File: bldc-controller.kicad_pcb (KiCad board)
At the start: 2 copper layers, 47 x 39 mm, 98 parts, among them IC1 L6205PD, P1 CON_LED, P10 MOUNTING, P11 CONN_01X03, P12 CONN_01X03, P2 MOUNTING, P3 CON_MOTOR, P4 USB_OTG, P5 CON_SWD, P6 CON_HALL, P7 CON_PWR_BRD, P8 MOUNTING, P9 MOUNTING, U1 STM32F405R, U5 MPU6000, U7 LD1117S33TR, Y1 Crystal

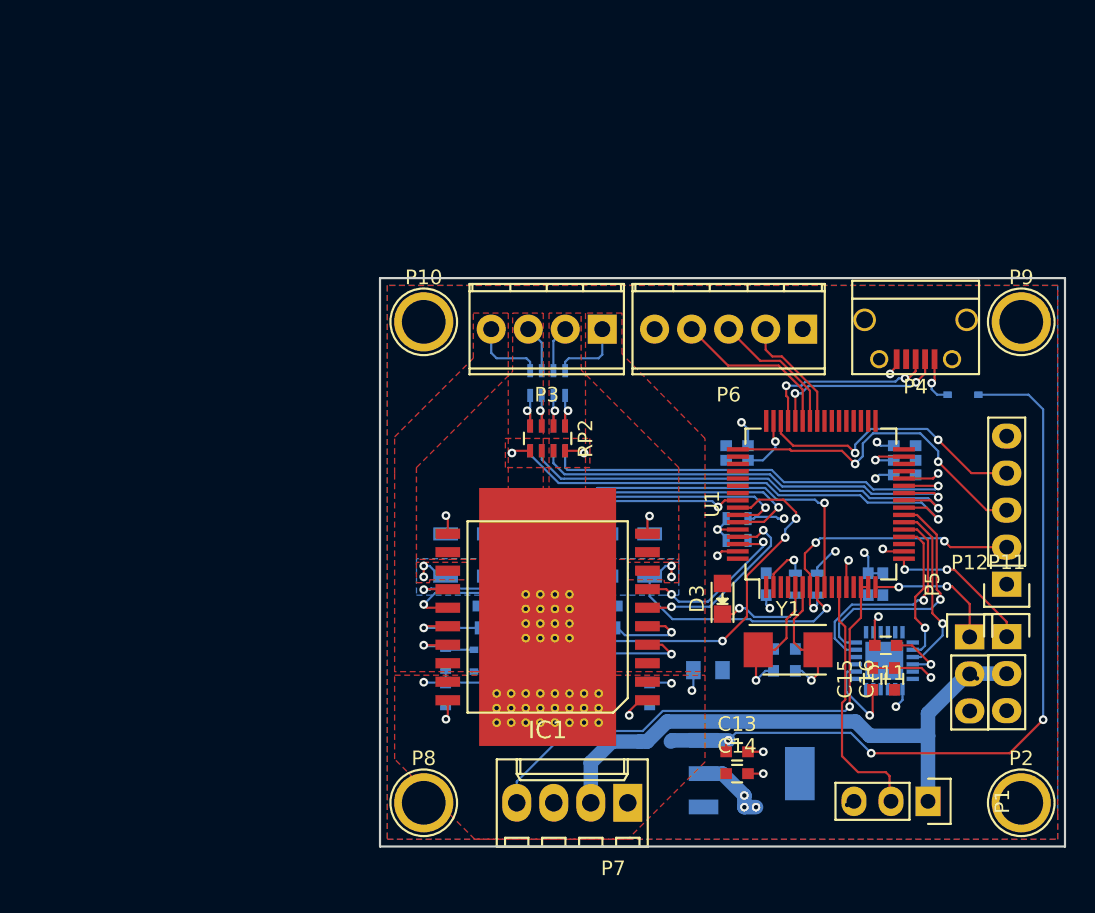
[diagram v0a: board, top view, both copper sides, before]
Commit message: routed... at least for now
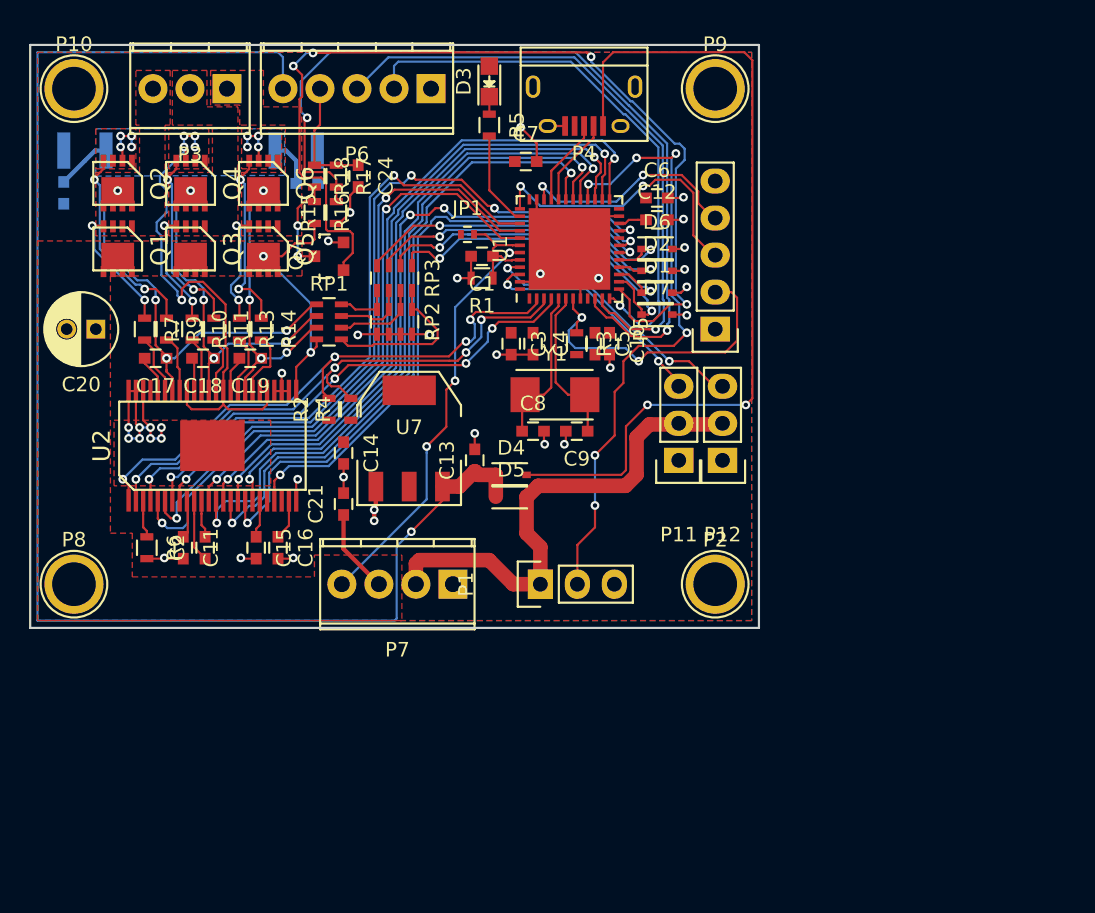
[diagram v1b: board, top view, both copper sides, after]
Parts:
- removed D8: D, Diodes_SMD:SOD-323
- removed IC1: L6205PD, BLDC:SOIC-20
- removed REF**1111111, REF**11111111111, REF**11111111112, REF**11111111113, REF**11111111114, REF**11111111121, REF**11111111122, REF**11111111123, REF**11111111124, REF**11111111131, REF**11111111132, REF**11111111133, REF**11111111134, REF**11111111141, REF**11111111142, REF**11111111143, REF**11111111144, REF**1111112, REF**1111113, REF**1111121, REF**1111122, REF**1111123, REF**1111131, REF**1111132, REF**1111133, REF**1111141, REF**1111142, REF**1111143, REF**1111151, REF**1111152, REF**1111153, REF**1111161, REF**1111162, REF**1111163, REF**1111171, REF**1111172, REF**1111173, REF**1111181, REF**1111182, REF**1111183: VIA-0.6, BLDC:VIA-0.6
- removed U5: MPU6000, Housings_DFN_QFN:QFN-24-1EP_4x4mm_Pitch0.5mm
- added C23: 1nF, Capacitors_SMD:C_0603, B.Cu at (119.0, 59.5)
- added C24: NA/100nF, Capacitors_SMD:C_0603, F.Cu at (122.5, 59.0)
- added D5: D_Small, Diodes_SMD:SOD-323, F.Cu at (133.0, 81.0)
- added D6: 3.3V, Diodes_SMD:SOD-323, F.Cu at (143.0, 64.0)
- added D7: 3.3V, Diodes_SMD:SOD-323, F.Cu at (143.0, 68.5)
- added JP1: OPEN, Resistors_SMD:R_0402, F.Cu at (130.0, 63.0)
- added Q1: Q_NMOS_DGS, BLDC:SOT1210, F.Cu at (106.0, 64.0)
- added Q2: Q_NMOS_DGS, BLDC:SOT1210, F.Cu at (106.0, 59.5)
- added Q3: Q_NMOS_DGS, BLDC:SOT1210, F.Cu at (111.0, 64.0)
- added Q4: Q_NMOS_DGS, BLDC:SOT1210, F.Cu at (111.0, 59.5)
- added Q5: Q_NMOS_DGS, BLDC:SOT1210, F.Cu at (116.0, 64.0)
- added Q6: Q_NMOS_DGS, BLDC:SOT1210, F.Cu at (116.0, 59.5)
- added Q7: 2N7002, TO_SOT_Packages_SMD:SOT-23, F.Cu at (120.5, 64.5)
- added R12: .01, Resistors_SMD:R_1210, B.Cu at (103.8, 57.2)
- added R13: 10R, Resistors_SMD:R_0603, F.Cu at (114.3, 69.5)
- added R14: 10R, Resistors_SMD:R_0603, F.Cu at (115.8, 69.5)
- added R15: NA/10kR, Resistors_SMD:R_0603, F.Cu at (121.0, 61.5)
- added R16: NA/10kR, Resistors_SMD:R_0603, F.Cu at (119.5, 61.5)
- added R17: 0R/50kR, Resistors_SMD:R_0603, F.Cu at (121.0, 59.0)
- added R18: NA/50kR, Resistors_SMD:R_0603, F.Cu at (119.5, 59.0)
- added U2: DRV8313, BLDC:SOIC-48, F.Cu at (112.5, 77.5)
- C1: value 220nF -> 100nF; moved to F.Cu
- C10, C12, C21, C3, C4, C5, C6, C7, C8, C9, D4, R5, U7: moved to F.Cu
- C11: value 100nF -> 2.2uF
- C17: value 2.2uF -> 100nF; moved to F.Cu
- C18, C19: value 2nF -> 100nF; moved to F.Cu
- C2: value 10nF -> 22nF; moved to F.Cu
- C20: value 100nF -> 10uF; footprint Capacitors_SMD:C_0603 -> Capacitors_ThroughHole:C_Radial_D5_L11_P2; moved to F.Cu
- C22: value 4.7uF -> 1nF; footprint Capacitors_SMD:C_0805 -> Capacitors_SMD:C_0603
- D1, D2: value D_Small -> 3.3V; moved to F.Cu
- P3: value CON_MOTOR -> CONN_01X03; footprint Terminal_Blocks:TerminalBlock_Pheonix_MPT-2.54mm_4pol -> Terminal_Blocks:TerminalBlock_Pheonix_MPT-2.54mm_3pol
- P7: footprint Connectors_Molex:Molex_KK-6410-04_04x2.54mm_Straight -> Terminal_Blocks:TerminalBlock_Pheonix_MPT-2.54mm_4pol
- R1: value 100 -> 10kR; moved to F.Cu
- R10, R11, R9: value .1 -> 10R; footprint Resistors_SMD:R_1206 -> Resistors_SMD:R_0603; moved to F.Cu
- R2: value NA -> 10kR; moved to F.Cu
- R3: value 0 -> 10kR; moved to F.Cu
- R4: value 10k -> 10kR; moved to F.Cu
- R6: value 10k -> 1R; moved to F.Cu
- R7: value 10k -> 10R; moved to F.Cu
- R8: value .1 -> .01; footprint Resistors_SMD:R_1206 -> Resistors_SMD:R_1210
- RP1: value 10k -> 20k; moved to F.Cu
- RP3: value 1k -> 10k; moved to F.Cu
- U1: value STM32F405R -> STM32F401CBUx; footprint Housings_QFP:TQFP-64_10x10mm_Pitch0.5mm -> Housings_DFN_QFN:QFN-48-1EP_7x7mm_Pitch0.5mm
- moved C22 55.0 mm to (102.3, 60.1), turned to 90 degrees
- moved C11 48.7 mm to (110.5, 84.5), turned to 270 degrees
- moved C20 45.5 mm to (104.5, 69.5), turned to 180 degrees
- moved C15 43.2 mm to (115.5, 84.5), turned to 270 degrees
- moved C16 43.2 mm to (117.0, 84.5), turned to 270 degrees
- moved C17 40.5 mm to (108.6, 71.5)
- moved D3 38.9 mm to (131.5, 52.5)
- moved R5 37.9 mm to (131.5, 55.5), turned to 270 degrees
- moved C7 37.3 mm to (134.0, 58.0), turned to 0 degrees
- moved R10 35.0 mm to (111.1, 69.5), turned to 270 degrees
- moved C14 34.8 mm to (121.5, 78.0), turned to 270 degrees
- moved R4 34.2 mm to (122.0, 75.0), turned to 90 degrees
- moved U7 32.9 mm to (126.0, 77.0), turned to 0 degrees
- moved R6 32.0 mm to (108.0, 84.5), turned to 270 degrees
- moved D4 31.5 mm to (133.0, 79.5), turned to 0 degrees
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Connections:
- net /OSC/OSC_IN renamed /OSC_IN
- net /OSC/OSC_OUT renamed /OSC_OUT
- C1 pad 1: Net-(C1-Pad1) -> /BOOT
- C1 pad 2: VPP -> GND
- C16 pad 1: VCC -> Net-(C16-Pad1)
- C17 pad 1: Net-(C17-Pad1) -> /DRV_OUT_1
- C17 pad 2: GND -> Net-(C17-Pad2)
- C18 pad 1: Net-(C18-Pad1) -> /DRV_OUT_2
- C18 pad 2: GND -> Net-(C18-Pad2)
- C19 pad 1: Net-(C19-Pad1) -> /DRV_OUT_3
- C19 pad 2: GND -> Net-(C19-Pad2)
- C22 pad 1: VPP -> GND
- C22 pad 2: GND -> Net-(C22-Pad2)
- D1 pad 1: Net-(D1-Pad1) -> /SENSE_V_3
- D1 pad 2: VPP -> GND
- D2 pad 1: Net-(C1-Pad1) -> /SENSE_V_2
- D2 pad 2: Net-(D1-Pad1) -> GND
- P1 pad 2: /CON_LED/LED_DATA -> /LED_MOSI
- P11 pad 1: /2CON/SIG_1 -> GND
- P11 pad 3: GND -> /PWM_2
- P12 pad 1: /2CON/SIG_2 -> GND
- P12 pad 3: GND -> /PWM_1
- P3 pad 1: /CON_MOTOR/C -> /DRV_OUT_3
- P3 pad 2: /CON_MOTOR/A -> /DRV_OUT_2
- P3 pad 3: /CON_MOTOR/B -> /DRV_OUT_1
- P4 pad 2: /USB/USB_DM -> /USB_D-
- P4 pad 3: /USB/USB_DP -> /USB_D+
- P5 pad 2: /SWDIO/NRST -> /NRST
- P5 pad 3: /SWDIO/SWDCLK -> /SWDCLK
- P5 pad 4: /SWDIO/SWDIO -> /SWDIO
- P6 pad 2: /HALL/HALL_W -> /HALL_W
- P6 pad 3: /HALL/HALL_V -> /HALL_V
- P6 pad 4: /HALL/HALL_U -> Net-(C24-Pad1)
- P6 pad 5: VCC -> +5V
- P7 pad 4: /Power/RX_TX_PWR_BOARD -> /COM_RX_TX_1
- R1 pad 1: Net-(C2-Pad2) -> /BOOT
- R1 pad 2: Net-(D1-Pad1) -> GND
- R10 pad 1: /driver/SENSE_A -> Net-(Q3-Pad2)
- R10 pad 2: GND -> Net-(R10-Pad2)
- R11 pad 1: /driver/SENSE_A -> Net-(Q4-Pad2)
- R11 pad 2: GND -> Net-(R11-Pad2)
- R2 pad 2: Net-(R2-Pad2) -> /DRV_NOCTW
- R3 pad 1: Net-(R2-Pad2) -> /NRST
- R3 pad 2: GND -> VCC
- R4 pad 2: /SWDIO/NRST -> /DRV_NFAULT
- R6 pad 1: Net-(C19-Pad1) -> Net-(R6-Pad1)
- R6 pad 2: /driver/EN_A -> GND
- R7 pad 1: Net-(C18-Pad1) -> Net-(Q1-Pad2)
- R7 pad 2: /driver/EN_B -> Net-(R7-Pad2)
- R8 pad 1: /driver/SENSE_B -> Net-(C22-Pad2)
- R9 pad 1: /driver/SENSE_B -> Net-(Q2-Pad2)
- R9 pad 2: GND -> Net-(R9-Pad2)
- RP1 pad 1: /CON_MOTOR/D -> /DRV_OUT_1
- RP1 pad 2: /CON_MOTOR/B -> /DRV_OUT_2
- RP1 pad 3: /CON_MOTOR/A -> /DRV_OUT_3
- RP1 pad 4: /CON_MOTOR/C -> VPP
- RP3 pad 1: /CUR_SENSE_4/OUT_4 -> /V_PP_SENSE
- RP3 pad 2: /CUR_SENSE_4/OUT_3 -> /SENSE_V_3
- RP3 pad 3: /CUR_SENSE_4/OUT_2 -> /SENSE_V_2
- RP3 pad 4: /CUR_SENSE_4/OUT_1 -> /SENSE_V_1
- U1 pad 10: (no net) -> /HALL_U
- U1 pad 11: /CON_LED/LED_DATA -> /HALL_V
- U1 pad 12: GND -> /HALL_W
- U1 pad 13: VCC -> /HALL_PWM
- U1 pad 14: /Power/RX_TX_PWR_BOARD -> /V_PP_SENSE
- U1 pad 15: /Power/RX_TX_PWR_BOARD -> /SENSE_V_3
- U1 pad 16: /2CON/SIG_2 -> /SENSE_V_2
- U1 pad 17: /2CON/SIG_1 -> /SENSE_V_1
- U1 pad 18: GND -> /CUR_SENSE_1
- U1 pad 19: VCC -> /DRV_L_C
- U1 pad 2: Net-(R5-Pad2) -> /DRV_NOCTW
- U1 pad 20: /IMU/nCS -> (no net)
- U1 pad 21: /IMU/SCK -> /DRV_DC_CAL
- U1 pad 22: /IMU/SDO -> Net-(C12-Pad1)
- U1 pad 23: /IMU/SDI -> GND
- U1 pad 24: /CUR_SENSE_4/OUT_1 -> VCC
- U1 pad 25: /CUR_SENSE_4/OUT_2 -> /DRV_ENABLE
- U1 pad 26: /CUR_SENSE_4/OUT_3 -> /DRV_L_A
- U1 pad 27: /CUR_SENSE_4/OUT_4 -> /DRV_L_B
- U1 pad 28: GND -> /LED_MOSI
- U1 pad 29: (no net) -> /DRV_H_A
- U1 pad 3: (no net) -> /DRV_NFAULT
- U1 pad 30: (no net) -> /DRV_H_B
- U1 pad 31: Net-(C12-Pad1) -> /DRV_H_C
- U1 pad 32: VCC -> /USB_D-
- U1 pad 33: (no net) -> /USB_D+
- U1 pad 34: (no net) -> /SWDIO
- U1 pad 35: (no net) -> GND
- U1 pad 36: (no net) -> VCC
- U1 pad 37: (no net) -> /SWDCLK
- U1 pad 38: (no net) -> Net-(R5-Pad2)
- U1 pad 39: (no net) -> /SPI_SCK
- U1 pad 4: (no net) -> /DRV_SPI_NCS
- U1 pad 40: (no net) -> /SPI_MISO
- U1 pad 41: /HALL/HALL_W -> /SPI_MOSI
- U1 pad 42: /HALL/HALL_V -> /BOOT
- U1 pad 43: /HALL/HALL_U -> /COM_RX_TX_1
- U1 pad 44: /USB/USB_DM -> /BOOT
- U1 pad 45: /USB/USB_DP -> /PWM_1
- U1 pad 46: /SWDIO/SWDIO -> /PWM_2
- U1 pad 47: Net-(C17-Pad1) -> GND
- U1 pad 49: /SWDIO/SWDCLK -> GND
- U1 pad 7: /SWDIO/NRST -> /NRST
- U1 pad 8: /driver/SENSE_A -> GND
- U1 pad 9: /driver/SENSE_B -> VCC
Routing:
- net /HALL_PWM: track 0.00 -> 65.8 mm, vias 0 -> 4
- net /HALL_U: track 0.00 -> 58.4 mm, vias 0 -> 2
- net Net-(D4-Pad2): track 3.40 -> 57.8 mm, vias 1 -> 2
- net Net-(C22-Pad2): track 0.00 -> 49.8 mm, vias 0 -> 13
- net /DRV_DC_CAL: track 0.00 -> 49.5 mm, vias 0 -> 4
- net /DRV_H_A: track 0.00 -> 48.7 mm, vias 0 -> 2
- net /DRV_ENABLE: track 0.00 -> 48.3 mm, vias 0 -> 2
- net /DRV_L_A: track 0.00 -> 46.4 mm, vias 0 -> 2
- net /DRV_H_B: track 0.00 -> 46.0 mm, vias 0 -> 2
- net /DRV_L_B: track 0.00 -> 44.8 mm, vias 0 -> 2
- net +5V: track 54.4 -> 99.0 mm, vias 3 -> 1
- net /SPI_MOSI: track 0.00 -> 44.2 mm, vias 0 -> 2
- net GND: track 25.7 -> 69.5 mm, vias 16 -> 35
- net /DRV_H_C: track 0.00 -> 43.7 mm, vias 0 -> 2
- net /DRV_L_C: track 0.00 -> 43.3 mm, vias 0 -> 4
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- added copper zone on F.Cu, net /DRV_OUT_1
- added copper zone on F.Cu, net /DRV_OUT_2
- added copper zone on F.Cu, net /DRV_OUT_3
- added copper zone on B.Cu, net Net-(C22-Pad2)
- added copper zone on F.Cu, net Net-(C22-Pad2)
- removed copper zone on F.Cu, net /CON_MOTOR/A
- removed copper zone on F.Cu, net /CON_MOTOR/B
- removed copper zone on F.Cu, net /CON_MOTOR/C
- removed copper zone on F.Cu, net /CON_MOTOR/D
- removed copper zone on B.Cu, net /driver/SENSE_A
- removed copper zone on F.Cu, net /driver/SENSE_A
- removed copper zone on B.Cu, net /driver/SENSE_B
- removed copper zone on F.Cu, net /driver/SENSE_B
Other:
- board size 47 x 39 mm -> 50 x 40 mm
- rule trace_min: 0.15 -> 0.1499
